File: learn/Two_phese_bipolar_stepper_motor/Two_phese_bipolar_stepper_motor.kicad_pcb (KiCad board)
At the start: 2 copper layers, 21 parts, among them J1 Screw_Terminal_01x02, J2 Screw_Terminal_01x02, J3 Screw_Terminal_01x12, J4 Screw_Terminal_01x04, U1 L297, U2 L298N

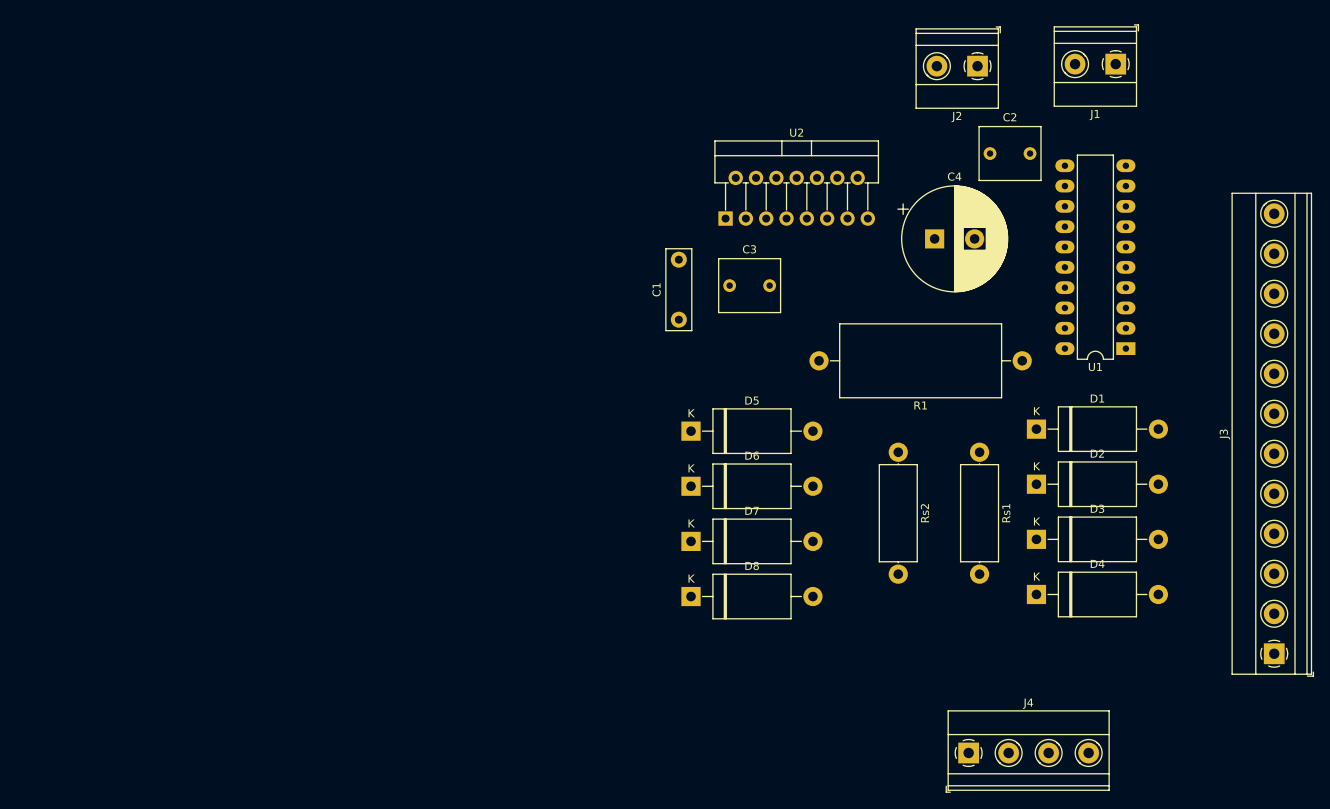
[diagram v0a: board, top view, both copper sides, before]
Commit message: 12/06/2023 make a pcb
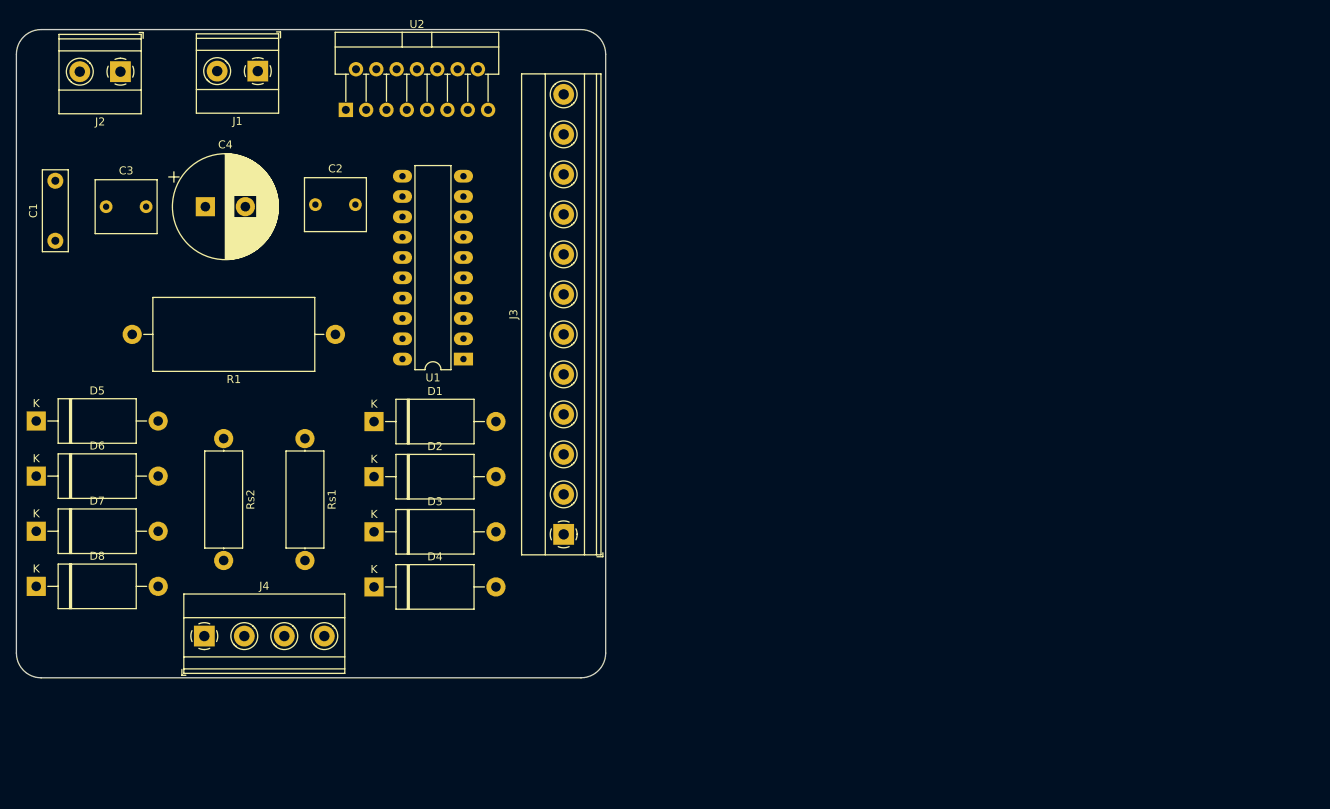
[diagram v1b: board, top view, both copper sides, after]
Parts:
- moved J1 107.2 mm to (143.2, 57.5)
- moved J2 107.1 mm to (126.0, 57.6)
- moved J4 96.7 mm to (136.5, 128.1)
- moved C4 91.2 mm to (136.7, 74.5)
- moved J3 90.1 mm to (181.4, 115.4)
- moved R1 85.9 mm to (152.9, 90.4)
- moved C2 84.6 mm to (150.4, 74.2)
- moved Rs2 84.3 mm to (138.9, 103.4)
- moved Rs1 84.3 mm to (149.1, 103.4)
- moved U1 82.8 mm to (168.9, 93.5)
- moved D1 82.8 mm to (157.7, 101.3)
- moved D2 82.8 mm to (157.7, 108.2)
- moved D3 82.8 mm to (157.7, 115.1)
- moved D4 82.8 mm to (157.7, 122.0)
- moved D5 81.9 mm to (115.5, 101.2)
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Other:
- board outline added: 73.7 x 81 mm
